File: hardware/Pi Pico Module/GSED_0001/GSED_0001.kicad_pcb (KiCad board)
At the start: 2 copper layers, 36 parts, among them J10 Ignition E-Match, J11 QD E-Match, J12 Radio, J13 Conn_01x20_Socket, J14 Power Input, J3 Conn_01x10_Socket (Digital), J4 K-Bottle PT, J5 Load Cell + Amp, J6 Tank PT, J7 Current Sensor, J8 K-Bottle TC, J9 Fill Servo, U1 BA90BC0FP-E2, U3 LMR33640ADDAR

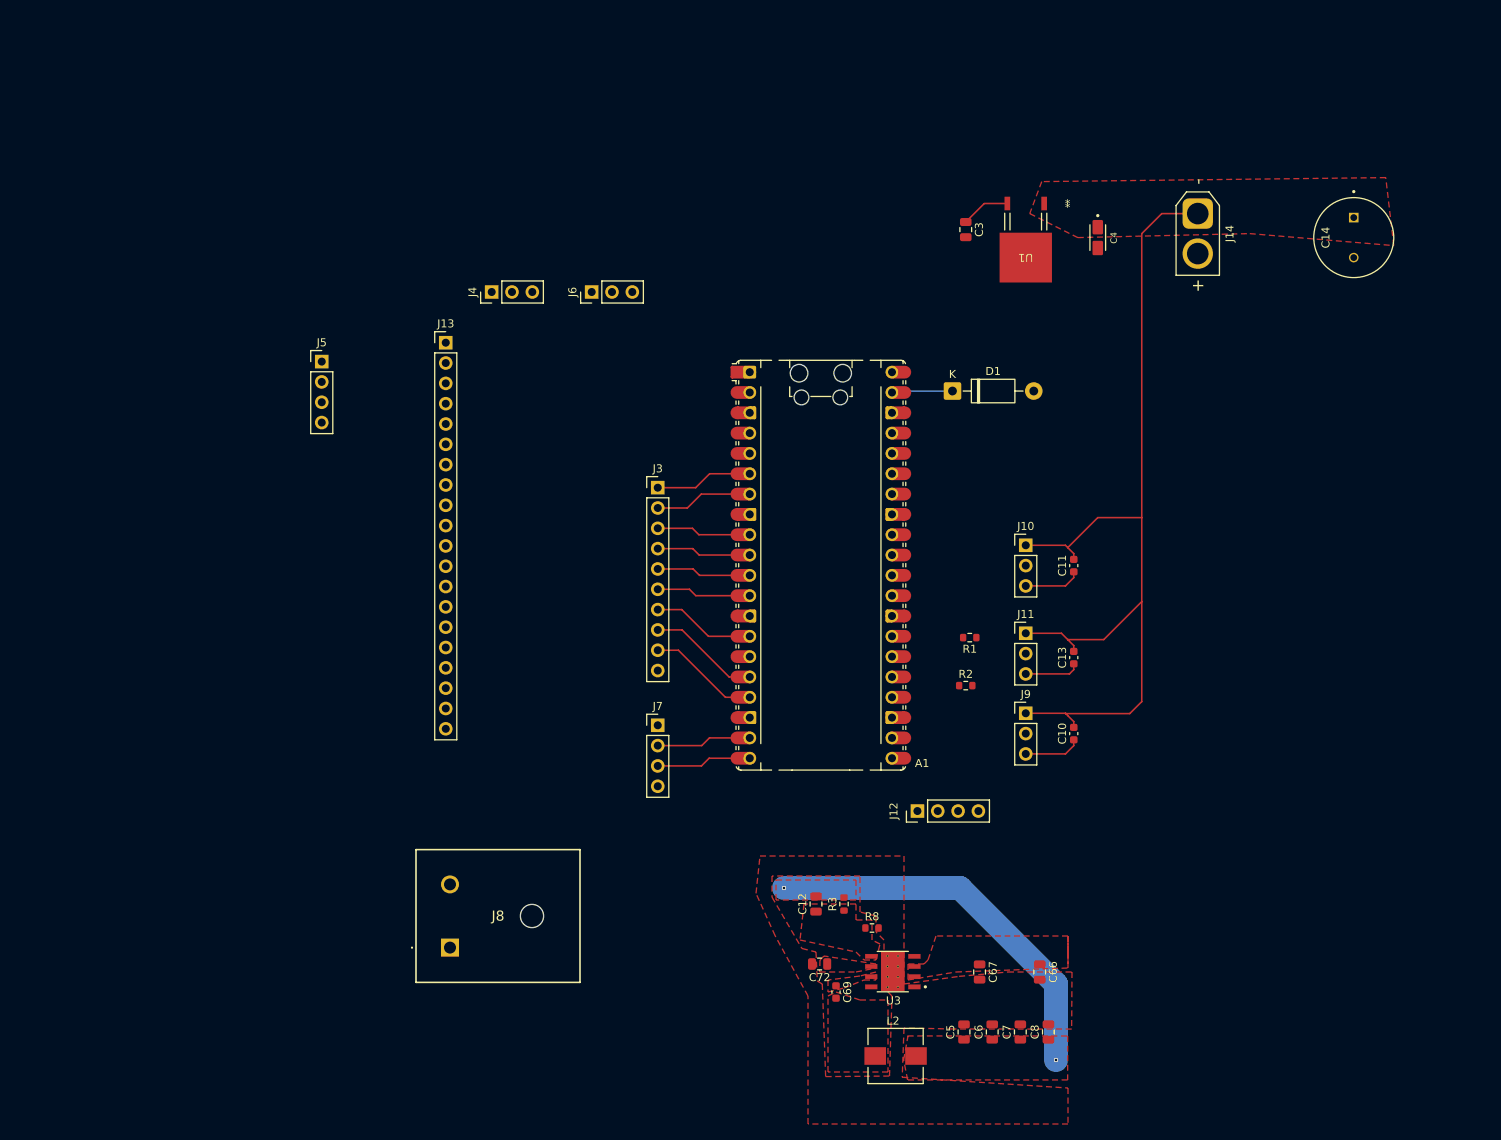
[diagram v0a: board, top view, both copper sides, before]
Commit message: Hopefully finished PCB
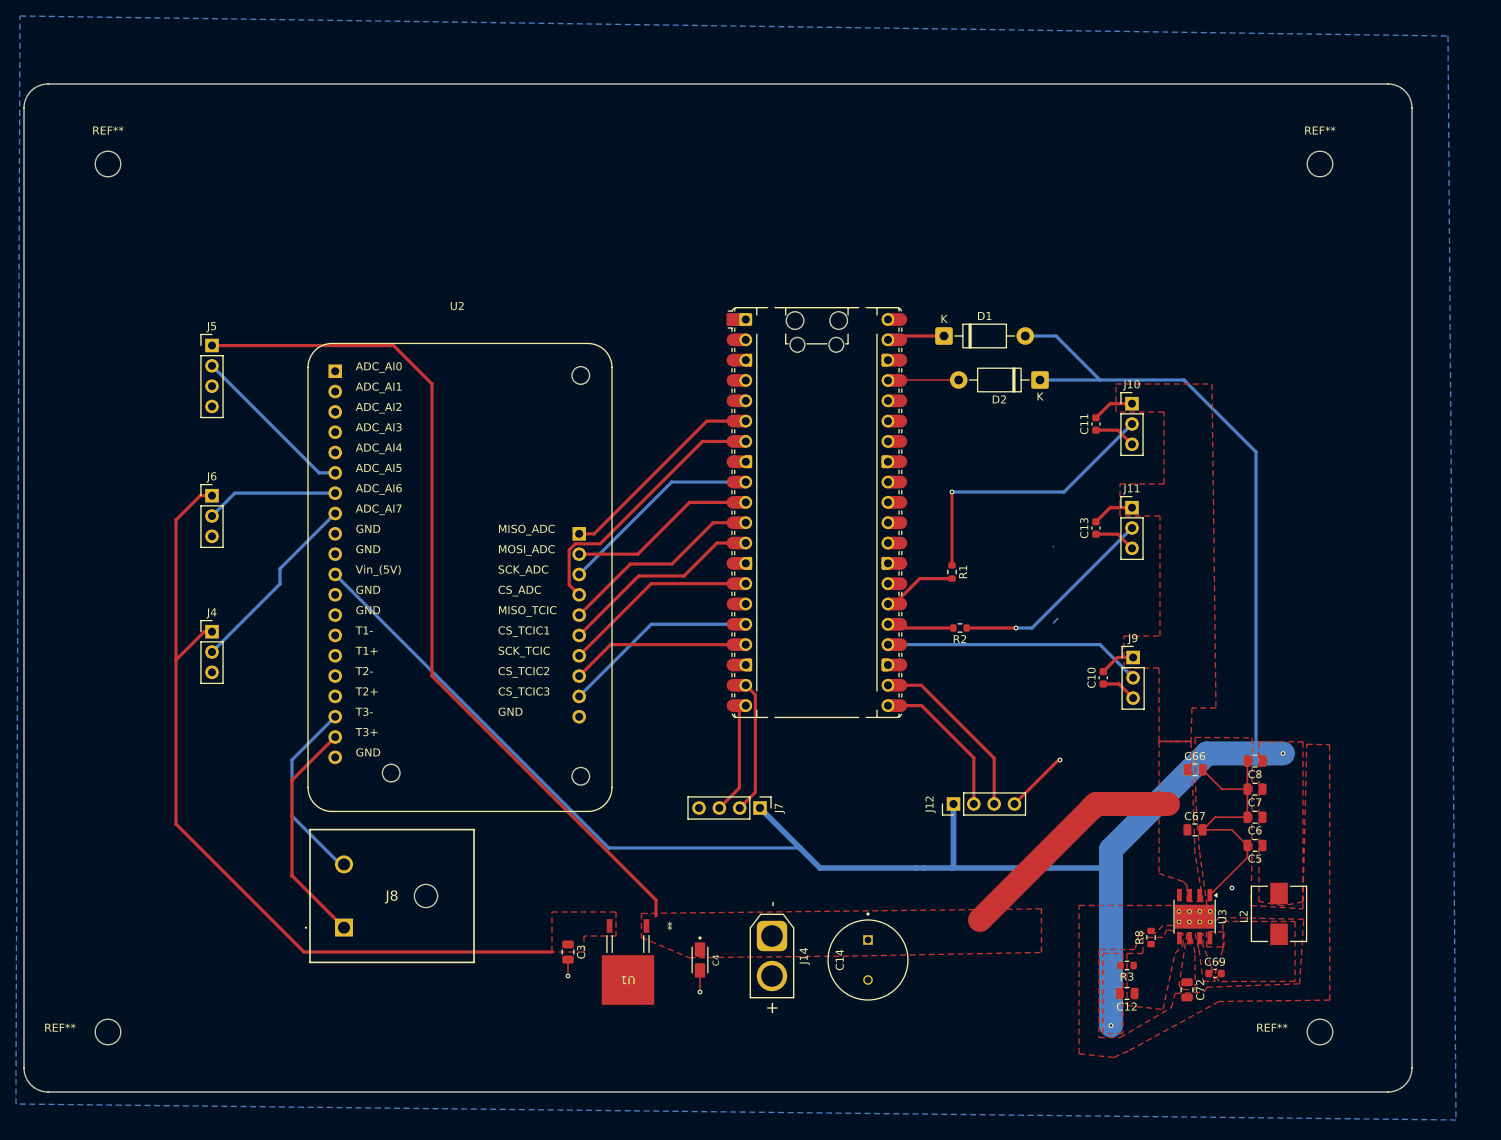
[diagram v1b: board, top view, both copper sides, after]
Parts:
- removed J13: Conn_01x20_Socket, Connector_PinHeader_2.54mm:PinHeader_1x20_P2.54mm_Vertical
- removed J3: Conn_01x10_Socket (Digital), Connector_PinHeader_2.54mm:PinHeader_1x10_P2.54mm_Vertical
- added D2: 1N5817, Diode_THT:D_DO-41_SOD81_P10.16mm_Horizontal, F.Cu at (177.0, 68.5)
- added REF**: MountingHole_3.2mm_M3, MountingHole:MountingHole_3.2mm_M3, F.Cu at (212.0, 150.0)
- added REF**: MountingHole_3.2mm_M3, MountingHole:MountingHole_3.2mm_M3, F.Cu at (212.0, 41.5)
- added REF**: MountingHole_3.2mm_M3, MountingHole:MountingHole_3.2mm_M3, F.Cu at (60.5, 41.5)
- added REF**: MountingHole_3.2mm_M3, MountingHole:MountingHole_3.2mm_M3, F.Cu at (60.5, 150.0)
- added U2: ~, DAQ_Module:DAQ_Module, F.Cu at (104.2, 59.8)
- U3: footprint LMR33640ADDAR:VREG_LM5017MR_NOPB -> Package_SO:Texas_HSOP-8-1EP_3.9x4.9mm_P1.27mm_ThermalVias
- moved C14 108.8 mm to (155.5, 141.0)
- moved J14 104.8 mm to (143.5, 138.0)
- moved C3 103.1 mm to (118.0, 140.0)
- moved C4 103.1 mm to (134.5, 141.0)
- moved U1 103.1 mm to (125.5, 143.5)
- moved J4 55.0 mm to (73.5, 100.0), turned to 0 degrees
- moved J6 53.9 mm to (73.5, 83.0), turned to 0 degrees
- moved L2 51.1 mm to (206.9, 135.2), turned to 90 degrees
- moved C69 47.4 mm to (198.9, 142.7), turned to 0 degrees
- moved C72 46.0 mm to (195.4, 144.7), turned to -90 degrees
- moved C5 43.2 mm to (203.9, 126.7), turned to 180 degrees
- moved C8 42.6 mm to (203.9, 116.1), turned to 180 degrees
- moved C6 42.4 mm to (203.9, 123.2), turned to 180 degrees
- moved C7 42.2 mm to (203.9, 119.6), turned to 180 degrees
- moved C12 40.5 mm to (187.9, 145.2), turned to 180 degrees
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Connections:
- A1 pad 37: +5V -> Net-(A1-3V3_EN)
- C66 pad 1: /BuckConverter/Vin (11.1V) -> +13V
- C67 pad 1: /BuckConverter/Vin (11.1V) -> +13V
- D1 pad 2: unconnected-(D1-A-Pad2) -> +5V
- U3 pad 2: /BuckConverter/Vin (11.1V) -> +13V
- U3 pad 3: /BuckConverter/Vin (11.1V) -> +13V
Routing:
- net +5V: track 48.5 -> 256.1 mm
- net +9V: track 6.16 -> 103.4 mm
- net GND: track 22.3 -> 62.9 mm, vias 0 -> 4
- net /GPIO20 (Ignition_E-Match): track 0.00 -> 35.2 mm, vias 0 -> 1
- net /GPIO18 (Fill Servo): track 0.00 -> 32.8 mm
- net +13V: track 120.4 -> 152.0 mm
- net /T+ (N2O): track 0.00 -> 28.8 mm
- net /GPIO19 (QD_E-Match): track 0.00 -> 25.9 mm, vias 0 -> 1
- net /ADC_AI0: track 0.00 -> 23.7 mm
- net /T- (N2O): track 0.00 -> 23.7 mm
- net /GPIO17 (UART_RX): track 0.00 -> 22.0 mm
- net /GPIO5 (CS_ADC): track 11.4 -> 33.0 mm
- net /ADC_AI2: track 0.00 -> 20.9 mm
- net /GPIO16 (UART_TX): track 0.00 -> 19.0 mm
- net /ADC_AI1: track 0.00 -> 16.6 mm
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- added copper zone on F.Cu, net +9V
- added copper zone on B.Cu, net GND
- removed copper zone on F.Cu, net /BuckConverter/Vin (11.1V)
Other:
- board outline added: 173.5 x 126 mm

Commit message: Done
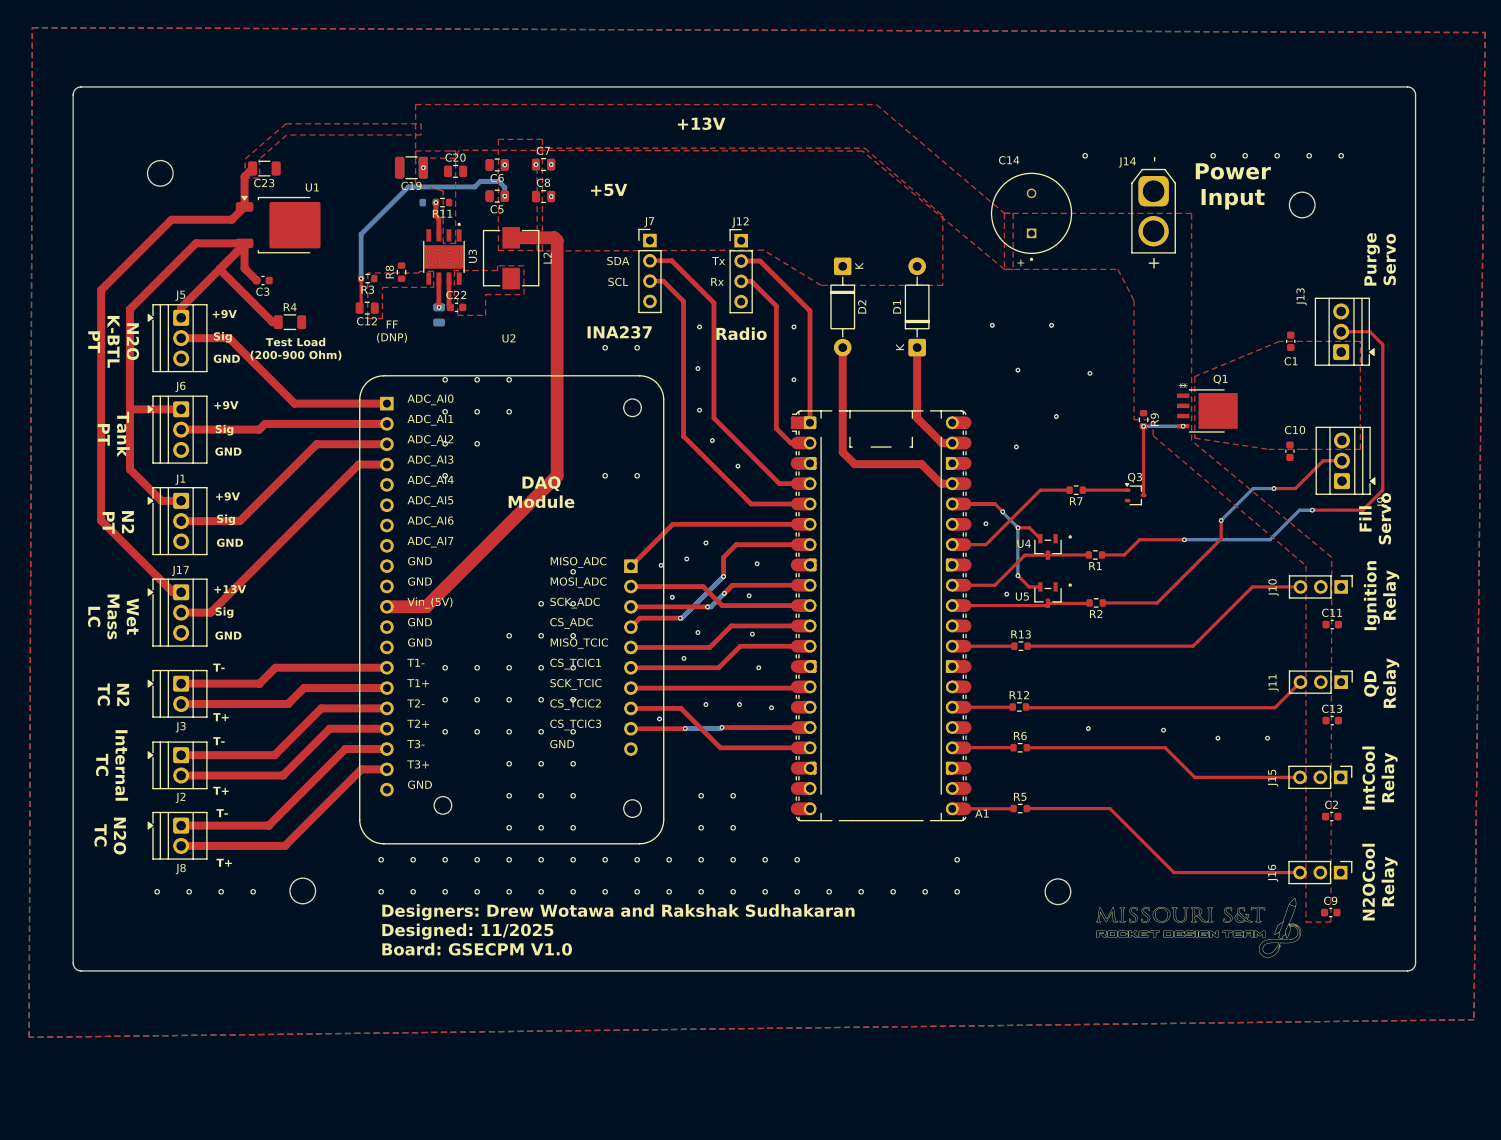
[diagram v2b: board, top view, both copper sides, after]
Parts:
- removed C4: 0.33 uF, TAJA334K050RNJ:CAPMP3216X180N
- removed C66: 10u, Capacitor_SMD:C_0805_2012Metric
- removed C67: 220n, Capacitor_SMD:C_0805_2012Metric
- removed C69: 100n, Capacitor_SMD:C_0603_1608Metric
- removed C72: 1u, Capacitor_SMD:C_0805_2012Metric
- removed J4: K-Bottle PT, Connector_PinHeader_2.54mm:PinHeader_1x03_P2.54mm_Vertical
- added C1: 100n, Capacitor_SMD:C_0603_1608Metric, F.Cu at (208.3, 63.7)
- added C15: 22 uF, Capacitor_SMD:C_0805_2012Metric, B.Cu at (109.2, 45.5)
- added C16: 22 uF, Capacitor_SMD:C_0805_2012Metric, B.Cu at (109.2, 41.6)
- added C17: 22 uF, Capacitor_SMD:C_0805_2012Metric, B.Cu at (114.9, 41.6)
- added C18: 10u, Capacitor_SMD:C_1210_3225Metric, B.Cu at (98.4, 41.9)
- added C19: 10u, Capacitor_SMD:C_1210_3225Metric, F.Cu at (98.4, 42.0)
- added C2: 100n, Capacitor_SMD:C_0603_1608Metric, F.Cu at (213.5, 123.1)
- added C20: 220n, Capacitor_SMD:C_0805_2012Metric, F.Cu at (104.0, 42.4)
- added C21: 1u, Capacitor_SMD:C_0805_2012Metric, B.Cu at (101.9, 60.4)
- added C22: 100n, Capacitor_SMD:C_0603_1608Metric, F.Cu at (104.1, 59.4)
- added C23: 0.33u, Capacitor_SMD:C_1206_3216Metric, F.Cu at (80.0, 42.1)
- added C9: 100n, Capacitor_SMD:C_0603_1608Metric, F.Cu at (213.3, 135.1)
- added G***: LOGO, RDT_Logo:RDT_Logo, F.Cu at (196.8, 137.0)
- added J1: N2-Bottle PT, TerminalBlock:TerminalBlock_Xinya_XY308-2.54-3P_1x03_P2.54mm_Horizontal, F.Cu at (69.6, 83.6)
- added J13: Purge Servo, TerminalBlock:TerminalBlock_Xinya_XY308-2.54-3P_1x03_P2.54mm_Horizontal, F.Cu at (214.6, 65.0)
- added J15: Internal Cooling, Connector_PinHeader_2.54mm:PinHeader_1x03_P2.54mm_Vertical, F.Cu at (214.6, 118.2)
- added J16: Nitrous Cooling, Connector_PinHeader_2.54mm:PinHeader_1x03_P2.54mm_Vertical, F.Cu at (214.6, 130.1)
- added J17: Load Cell + Amp, TerminalBlock:TerminalBlock_Xinya_XY308-2.54-3P_1x03_P2.54mm_Horizontal, F.Cu at (69.6, 95.0)
- added J2: K-Bottle TC, TerminalBlock:TerminalBlock_Xinya_XY308-2.54-2P_1x02_P2.54mm_Horizontal, F.Cu at (69.6, 115.4)
- added J3: K-Bottle TC, TerminalBlock:TerminalBlock_Xinya_XY308-2.54-2P_1x02_P2.54mm_Horizontal, F.Cu at (69.6, 106.5)
- added Q1: BUK6Y33-60PX, BUK6Y33-60PX:LFPAK_SOT669_NEX, F.Cu at (197.8, 72.4)
- added Q3: Q_NPN, Package_TO_SOT_SMD:SOT-323_SC-70, F.Cu at (188.9, 82.9)
- added R10: 2.49k, Resistor_SMD:R_0603_1608Metric, B.Cu at (100.7, 46.3)
- added R11: 10K, Resistor_SMD:R_0603_1608Metric, F.Cu at (102.3, 46.3)
- added R12: 2.49k, Resistor_SMD:R_0603_1608Metric, F.Cu at (174.4, 109.4)
- added R13: 2.49k, Resistor_SMD:R_0603_1608Metric, F.Cu at (174.6, 101.8)
- added R4: 1k, Resistor_SMD:R_1206_3216Metric, F.Cu at (83.2, 61.3)
- added R5: 2.49k, Resistor_SMD:R_0603_1608Metric, F.Cu at (174.5, 122.1)
- added R6: 2.49k, Resistor_SMD:R_0603_1608Metric, F.Cu at (174.5, 114.5)
- added R7: 10K, Resistor_SMD:R_0603_1608Metric, F.Cu at (181.5, 82.3)
- added R9: 10K, Resistor_SMD:R_0603_1608Metric, F.Cu at (189.9, 73.5)
- added U4: BAV199_215, BAV199_215:TO-236AB_NEX, F.Cu at (178.0, 89.4)
- added U5: BAV199_215, BAV199_215:TO-236AB_NEX, F.Cu at (178.0, 95.4)
- C3: value 22 uF -> 100n; footprint Capacitor_SMD:C_0805_2012Metric -> Capacitor_SMD:C_0603_1608Metric
- J12: value Radio -> Radio Module Connector
- J5: value Load Cell + Amp -> K-Bottle PT; footprint Connector_PinHeader_2.54mm:PinHeader_1x04_P2.54mm_Vertical -> TerminalBlock:TerminalBlock_Xinya_XY308-2.54-3P_1x03_P2.54mm_Horizontal
- J6, J9: footprint Connector_PinHeader_2.54mm:PinHeader_1x03_P2.54mm_Vertical -> TerminalBlock:TerminalBlock_Xinya_XY308-2.54-3P_1x03_P2.54mm_Horizontal
- J8: footprint AM-K-PCB:AMKPCB -> TerminalBlock:TerminalBlock_Xinya_XY308-2.54-2P_1x02_P2.54mm_Horizontal
- U1: value BA90BC0FP-E2 -> L78M09CDT-TR; footprint BA90BC0FP_E2:TO252-3_ROM -> Package_TO_SOT_SMD:TO-252-2
- U2: value ~ -> DAQ_Module
- U3: footprint Package_SO:Texas_HSOP-8-1EP_3.9x4.9mm_P1.27mm_ThermalVias -> LMR33640ADDAR:VREG_LM5017MR_NOPB
- moved R3 128.0 mm to (93.0, 55.8)
- moved C12 127.9 mm to (92.9, 59.5)
- moved L2 126.2 mm to (110.9, 53.3)
- moved R8 125.3 mm to (97.2, 55.0)
- moved C6 125.0 mm to (109.2, 41.6)
- moved U3 124.9 mm to (102.5, 53.1)
- moved C5 124.7 mm to (109.2, 45.5)
- moved C7 118.3 mm to (114.9, 41.6), turned to 0 degrees
- moved C8 113.5 mm to (114.9, 45.6), turned to 0 degrees
- moved J14 104.6 mm to (191.2, 44.9)
- moved U1 103.6 mm to (82.6, 49.1), turned to 0 degrees
- moved C14 95.5 mm to (175.9, 47.7), turned to 90 degrees
- moved C3 92.2 mm to (79.9, 56.1), turned to 180 degrees
- moved J12 75.2 mm to (139.6, 51.1), turned to 0 degrees
- moved J7 72.3 mm to (128.2, 51.1), turned to 0 degrees
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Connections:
- net /GPIO13 (CSChamberShell_2) renamed /GPIO13 (CS_Internal)
- net /GPIO9 (CSChamberShell_1) renamed /GPIO9 (CS_N2)
- net Net-(U3-FB) renamed /BuckConverter/FB
- net Net-(U3-SW) renamed /BuckConverter/SW
- A1 pad 1: unconnected-(A1-GPIO0-Pad1) -> /GPIO0 (Radio_UART_TX)
- A1 pad 19: /GPIO14_INA237 SDA -> unconnected-(A1-GPIO14-Pad19)_1
- A1 pad 2: unconnected-(A1-GPIO1-Pad2) -> /GPIO1 (Radio_UART_RX)
- A1 pad 20: /GPIO15_INA237 SCL -> unconnected-(A1-GPIO15-Pad20)_1
- A1 pad 21: /GPIO16 (UART_TX) -> /GPIO16 (Nitrous_Cooling)
- A1 pad 22: /GPIO17 (UART_RX) -> unconnected-(A1-GPIO17-Pad22)_1
- A1 pad 24: /GPIO18 (Fill Servo) -> /GPIO18 (Internal_Cooling)
- A1 pad 25: Net-(A1-GPIO19) -> unconnected-(A1-GPIO19-Pad25)_1
- A1 pad 26: Net-(A1-GPIO20) -> /GPIO20 (QD_E-Match)
- A1 pad 29: unconnected-(A1-GPIO22-Pad29) -> /GPIO22 (Ignition_E-Match)
- A1 pad 31: unconnected-(A1-GPIO26_ADC0-Pad31) -> Net-(A1-GPIO26_ADC0)
- A1 pad 32: unconnected-(A1-GPIO27_ADC1-Pad32) -> Net-(A1-GPIO27_ADC1)
- A1 pad 33: unconnected-(A1-AGND-Pad33) -> GND
- A1 pad 34: unconnected-(A1-GPIO28_ADC2-Pad34) -> /GPIO28 (ServoPWR_Switch)
- A1 pad 36: unconnected-(A1-3V3-Pad36) -> +3.3V
- A1 pad 4: unconnected-(A1-GPIO2-Pad4) -> /GPIO2_INA237 SDA
- A1 pad 5: unconnected-(A1-GPIO3-Pad5) -> /GPIO3_INA237 SCL
- C10 pad 1: GND -> +V_Servo
- C10 pad 2: +13V -> GND
- C11 pad 1: GND -> +13V
- C11 pad 2: +13V -> GND
- C13 pad 1: GND -> +13V
- C13 pad 2: +13V -> GND
- C3 pad 1: +9V -> GND
- C3 pad 2: GND -> +9V
- J10 pad 1: +13V -> GND
- J10 pad 2: /GPIO20 (Ignition_E-Match) -> +13V
- J10 pad 3: GND -> Net-(J10-Pin_3)
- J11 pad 1: +13V -> GND
- J11 pad 2: /GPIO19 (QD_E-Match) -> +13V
- J11 pad 3: GND -> Net-(J11-Pin_3)
- J12 pad 2: /GPIO16 (UART_TX) -> /GPIO0 (Radio_UART_TX)
- J12 pad 3: /GPIO17 (UART_RX) -> /GPIO1 (Radio_UART_RX)
- J14 pad 1: +13V -> GND
- J14 pad 2: GND -> +13V
- J5 pad 1: +13V -> +9V
- J5 pad 2: /ADC_AI2 -> /ADC_AI0
- J5 pad 3: unconnected-(J5-Pin_3-Pad3) -> GND
- J7 pad 2: /GPIO14_INA237 SDA -> /GPIO2_INA237 SDA
- J7 pad 3: /GPIO15_INA237 SCL -> /GPIO3_INA237 SCL
- J8 pad 1: /T+ (N2O) -> /T- (N2O)
- J8 pad 2: /T- (N2O) -> /T+ (N2O)
- J9 pad 1: +13V -> GND
- J9 pad 2: /GPIO18 (Fill Servo) -> /GPIO26 (Fill Servo)
- J9 pad 3: GND -> +V_Servo
- R1 pad 1: /GPIO20 (Ignition_E-Match) -> /GPIO27 (Purge Servo)
- R1 pad 2: Net-(A1-GPIO20) -> Net-(A1-GPIO27_ADC1)
- R2 pad 1: /GPIO19 (QD_E-Match) -> /GPIO26 (Fill Servo)
- R2 pad 2: Net-(A1-GPIO19) -> Net-(A1-GPIO26_ADC0)
- U1 pad 2: unconnected-(U1-N.C./GND-Pad2) -> GND
- U2 pad 1: /ADC_AI7 -> /ADC_AI0
- U2 pad 14: /T- (ChamberShell_1) -> /T- (N2)
- U2 pad 15: /T+ (ChamberShell_1) -> /T+ (N2)
- U2 pad 16: /T- (ChamberShell_2) -> /T- (Internal)
- U2 pad 17: /T+ (ChamberShell_2) -> /T+ (Internal)
- U2 pad 2: /ADC_AI6 -> /ADC_AI1
- U2 pad 3: /ADC_AI5 -> /ADC_AI2
- U2 pad 4: /ADC_AI4 -> /ADC_AI3
- U2 pad 5: /ADC_AI3 -> unconnected-(U2-ADC_AI4-Pad5)
- U2 pad 6: /ADC_AI2 -> unconnected-(U2-ADC_AI5-Pad6)
- U2 pad 7: /ADC_AI1 -> unconnected-(U2-ADC_AI6-Pad7)
- U2 pad 8: /ADC_AI0 -> unconnected-(U2-ADC_AI7-Pad8)
- U3 pad 3: +13V -> Net-(U3-EN)
- U3 pad 9: (no net) -> GND
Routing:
- net +5V: track 256.1 -> 94.8 mm, vias 2 -> 4
- net +13V: track 152.0 -> 70.0 mm, vias 0 -> 1
- net GND: track 62.9 -> 0.00 mm, vias 4 -> 126
- net /GPIO27 (Purge Servo): track 0.00 -> 62.5 mm, vias 0 -> 2
- net /GPIO3_INA237 SCL: track 0.00 -> 41.4 mm
- net /GPIO2_INA237 SDA: track 0.00 -> 40.0 mm
- net /GPIO26 (Fill Servo): track 0.00 -> 38.6 mm, vias 0 -> 2
- net Net-(J16-Pin_3): track 0.00 -> 37.5 mm
- net Net-(J10-Pin_3): track 0.00 -> 37.2 mm
- net Net-(J15-Pin_3): track 0.00 -> 35.7 mm
- net Net-(J11-Pin_3): track 0.00 -> 35.7 mm
- net /GPIO20 (Ignition_E-Match): track 35.2 -> 0.00 mm, vias 1 -> 0
- net /ADC_AI3: track 0.00 -> 33.4 mm
- net /GPIO18 (Fill Servo): track 32.8 -> 0.00 mm
- net /T- (Internal): track 0.00 -> 28.1 mm
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- added copper zone on F.Cu, net +V_Servo
- removed copper zone on F.Cu, net +9V
- removed copper zone on F.Cu, net Net-(U3-BOOT)
- removed copper zone on F.Cu, net Net-(U3-VCC)
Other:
- board size 173.5 x 126 mm -> 167.8 x 110.5 mm
- board text added: "+13V"
- board text added: "+5V"
- board text added: "+9V"
- board text added: "DAQ Module"
- board text added: "Designers: Drew Wotawa and Rakshak Sudhakaran Designed: 11/2025 Board: GSECPM V1.0"
- board text added: "FF (DNP)"
- board text added: "Fill Servo"
- board text added: "GND"
- board text added: "INA237"
- board text added: "Ignition Relay"
- board text added: "IntCool Relay"
- board text added: "Internal TC"
- board text added: "N2 PT"
- board text added: "N2 TC"
- board text added: "N2O K-BTL PT"
- board text added: "N2O TC"
- board text added: "N2OCool Relay"
- board text added: "Power Input"
- board text added: "Purge Servo"
- board text added: "QD Relay"
- board text added: "Radio"
- board text added: "Rx"
- board text added: "SCL"
- board text added: "SDA"
- board text added: "Sig"
- board text added: "T+"
- board text added: "T-"
- board text added: "Tank PT"
- board text added: "Test Load (200-900 Ohm)"
- board text added: "Tx"
- board text added: "Wet Mass LC"
- board text added: "{ "ViaStitching": "0.2", "stitch_zone_0": { "HSpacing": "2", "VSpacing": "2", "HOffset": "0", "VOffset": "0", "Clearance": "2", "Randomize": false } }"
- board text added: "{ "ViaStitching": "0.2", "stitch_zone_0": { "HSpacing": "3", "VSpacing": "3", "HOffset": "0", "VOffset": "0", "Clearance": "3", "Randomize": false } }"
- board text added: "{ "ViaStitching": "0.2", "stitch_zone_0": { "HSpacing": "4", "VSpacing": "4", "HOffset": "0", "VOffset": "0", "Clearance": "4", "Randomize": false } }"
- board text added: "{ "ViaStitching": "0.2", "stitch_zone_0": { "HSpacing": "4", "VSpacing": "4", "HOffset": "0", "VOffset": "0", "Clearance": "4", "Randomize": true } }"
- board text added: "{ "ViaStitching": "0.2", "stitch_zone_0": { "HSpacing": "5", "VSpacing": "5", "HOffset": "0", "VOffset": "0", "Clearance": "5", "Randomize": false } }"
- board text added: "{ "ViaStitching": "0.2", "stitch_zone_0": { "HSpacing": "5", "VSpacing": "5", "HOffset": "0", "VOffset": "0", "Clearance": "5", "Randomize": true } }"
